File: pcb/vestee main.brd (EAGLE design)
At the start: 65 x 65 mm, 54 parts, among them IC1 LD117AS12TR, IC2 FT232RL, Q1 MMBT2222A, Q2 MMBT5088, Q3 MMBT4403, Q4 MMBT5088, Q5 MMBT5088

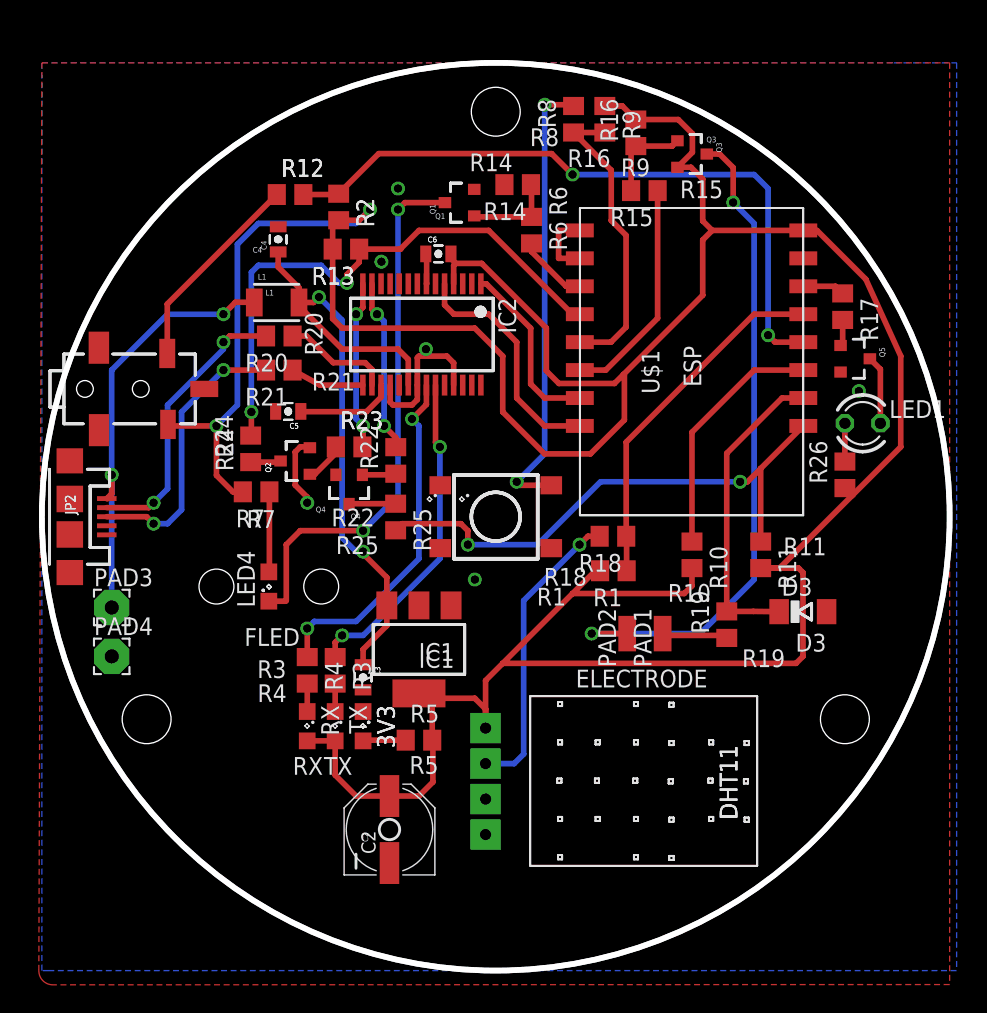
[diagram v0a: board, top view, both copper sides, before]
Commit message: Version 2, all issues fixed
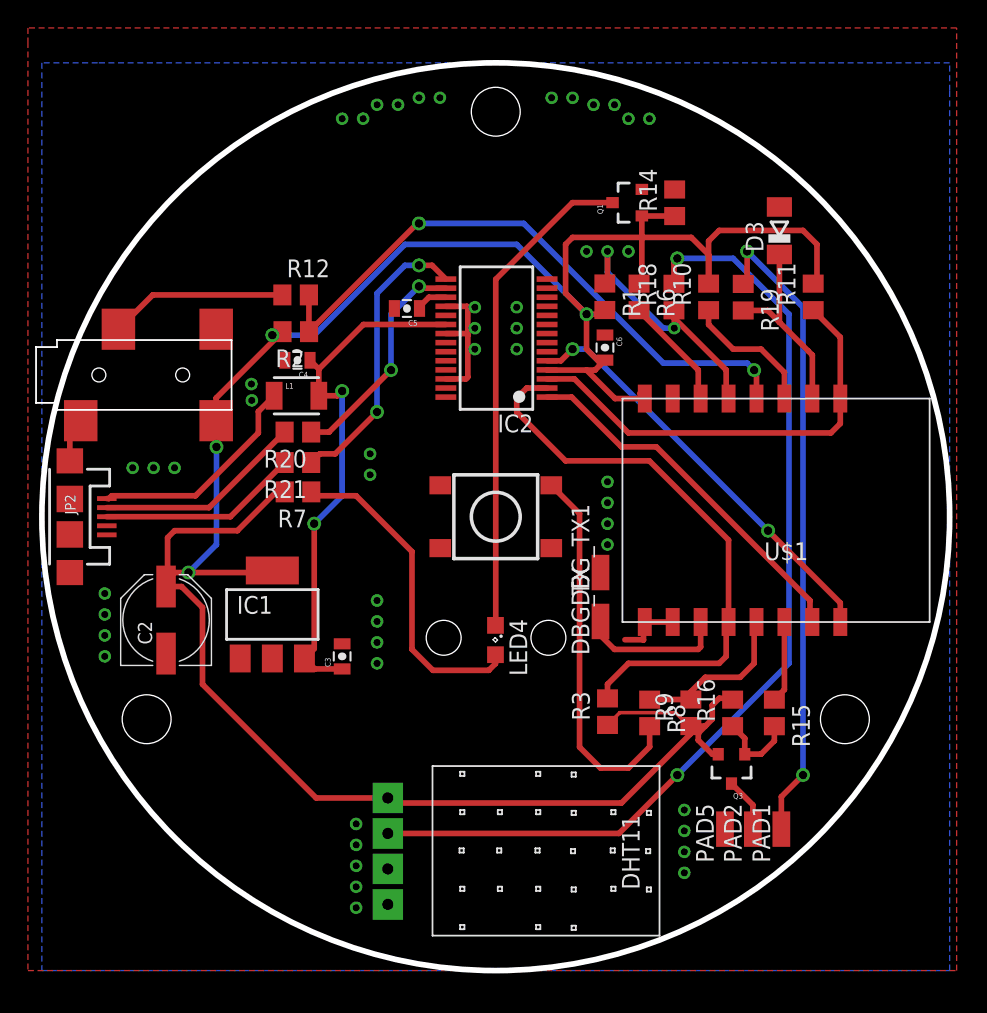
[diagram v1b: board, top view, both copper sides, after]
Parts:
- removed 3V3, RX, TX: (no value), led:SML0805
- removed LED1: (no value), led:LED3MM
- removed PAD3, PAD4: WIREPAD2,54/1,0, wirepad:2,54/1,0
- removed Q2, Q4, Q5: MMBT5088, SparkFun-DiscreteSemi:SOT23-3
- removed R13, R17, R22, R23, R24, R25, R26, R4, R5: (no value), rcl:R0805
- added DBG_TX, DBG_TX1, PAD5: (no value), wirepad:SMD1,27-2,54
- PRPIHERALS: value (none) -> AUDIO-JACK-2.5-CUI; device SparkFun-Connectors:STEREOJACK2.5MM -> SparkFun-Connectors:STEREOJACK2.5_SMD_CUI
- moved Q3 44.1 mm to (49.4, 14.5), turned to 180 degrees
- moved R9 42.9 mm to (46.5, 18.5), turned to 90 degrees
- moved R8 42.9 mm to (43.5, 18.4), turned to 270 degrees
- moved R16 42.1 mm to (49.5, 18.4)
- moved R15 38.5 mm to (52.5, 18.4), turned to 270 degrees
- moved D3 27.3 mm to (52.8, 53.0), turned to 90 degrees
- moved R19 23.5 mm to (50.2, 48.2), turned to 270 degrees
- moved C2 21.9 mm to (8.89, 25.1)
- moved R3 19.7 mm to (40.5, 18.5), turned to 90 degrees
- moved R1 19.6 mm to (40.3, 48.2), turned to 270 degrees
- moved R11 18.8 mm to (55.2, 48.2), turned to 90 degrees
- moved R10 18.5 mm to (47.7, 48.2), turned to 90 degrees
- moved R18 17.7 mm to (45.3, 48.2), turned to 90 degrees
- moved LED4 16.7 mm to (32.5, 23.7), turned to 270 degrees
- moved PAD2 16.6 mm to (50.9, 10.1)
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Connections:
- removed net CBUS: R13.1, R24.2, U$1.GPIO0
- removed net CBUS_RST: R11.1, R25.2, U$1.REST
- removed net N$11: IC2.23, R3.1
- removed net N$12: IC2.22, R4.1
- removed net N$13: R3.2, TX.C
- removed net N$14: R4.2, RX.C
- removed net N$20: R17.1, U$1.GPIO12
- removed net N$22: LED1.K, Q5.3
- removed net N$23: LED1.A, R26.2
- removed net N$30: IC2.13, R22.2
- removed net N$31: Q2.3, R24.1
- removed net N$32: Q2.1, R23.1
- removed net N$33: Q4.1, R22.1
- removed net N$34: IC2.14, R23.2
- removed net N$35: Q4.3, R25.1
- removed net N$8: 3V3.A, R5.1
- new net DTR: IC2.2, R3.2, U$1.GPIO0
- new net RTS: IC2.3, R11.1, U$1.REST
- net 1-WIRE: now also PRPIHERALS.3; no longer PRPIHERALS.1
- net FLED: now also U$1.GPIO12; no longer U$1.GPIO2
- net GND: now also DBG_TX1.1, PAD5.1, PRPIHERALS.1; no longer 3V3.C, PAD4.1, PRPIHERALS.5, Q2.2, Q4.2, Q5.2
- net N$5: now also DBG_TX.1, U$1.GPIO2; no longer Q5.1, R17.2
- net N$7: no longer PAD3.1
- net VCC: now also PRPIHERALS.2, R3.1; no longer PRPIHERALS.4, R13.2, R26.1, R5.2, RX.A, TX.A
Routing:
- net VCC: track 245.3 -> 182.1 mm, vias 2 -> 4
- net N$6: track 21.4 -> 70.4 mm, vias 1 -> 2
- net N$17: track 48.2 -> 3.89 mm, vias 2 -> 0
- net N$26: track 4.72 -> 46.1 mm, vias 0 -> 2
- net DTR: track 0.00 -> 41.2 mm
- net CBUS: track 40.9 -> 0.00 mm, vias 2 -> 0
- net CBUS_RST: track 39.3 -> 0.00 mm, vias 2 -> 0
- net RTS: track 0.00 -> 31.8 mm
- net N$12: track 25.2 -> 0.00 mm, vias 2 -> 0
- net N$11: track 23.6 -> 0.00 mm, vias 2 -> 0
- net N$15: track 5.75 -> 23.4 mm
- net N$28: track 5.31 -> 20.9 mm, vias 0 -> 2
- net N$7: track 31.2 -> 15.9 mm, vias 2 -> 0
- net FTDI_TXD: track 12.8 -> 26.5 mm
- net FTDI_RXD: track 17.1 -> 30.2 mm, vias 0 -> 2
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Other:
- board text removed: "/Users/grzegorz/Documents/montebmp.bmp"
- board text removed: "3V3"
- board text removed: "C2"
- board text removed: "C3"
- board text removed: "C4"
- board text removed: "C5"
- board text removed: "C6"
- board text removed: "D3"
- board text removed: "DHT11"
- board text removed: "ELECTRODE"
- board text removed: "ESP"
- board text removed: "FLED"
- board text removed: "IC1"
- board text removed: "JP2"
- board text removed: "L1"
- board text removed: "Q1"
- board text removed: "Q2"
- board text removed: "Q3"
- board text removed: "Q4"
- board text removed: "R1"
- board text removed: "R10"
- board text removed: "R11"
- board text removed: "R12"
- board text removed: "R13"
- board text removed: "R14"
- board text removed: "R15"
- board text removed: "R16"
- board text removed: "R18"
- board text removed: "R19"
- board text removed: "R2"
- board text removed: "R20"
- board text removed: "R21"
- board text removed: "R22"
- board text removed: "R23"
- board text removed: "R24"
- board text removed: "R25"
- board text removed: "R3"
- board text removed: "R4"
- board text removed: "R5"
- board text removed: "R6"
- board text removed: "R7"
- board text removed: "R8"
- board text removed: "R9"
- board text removed: "RX"
- board text removed: "TX"
- board text removed: "vestee"

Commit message: pcb rev3
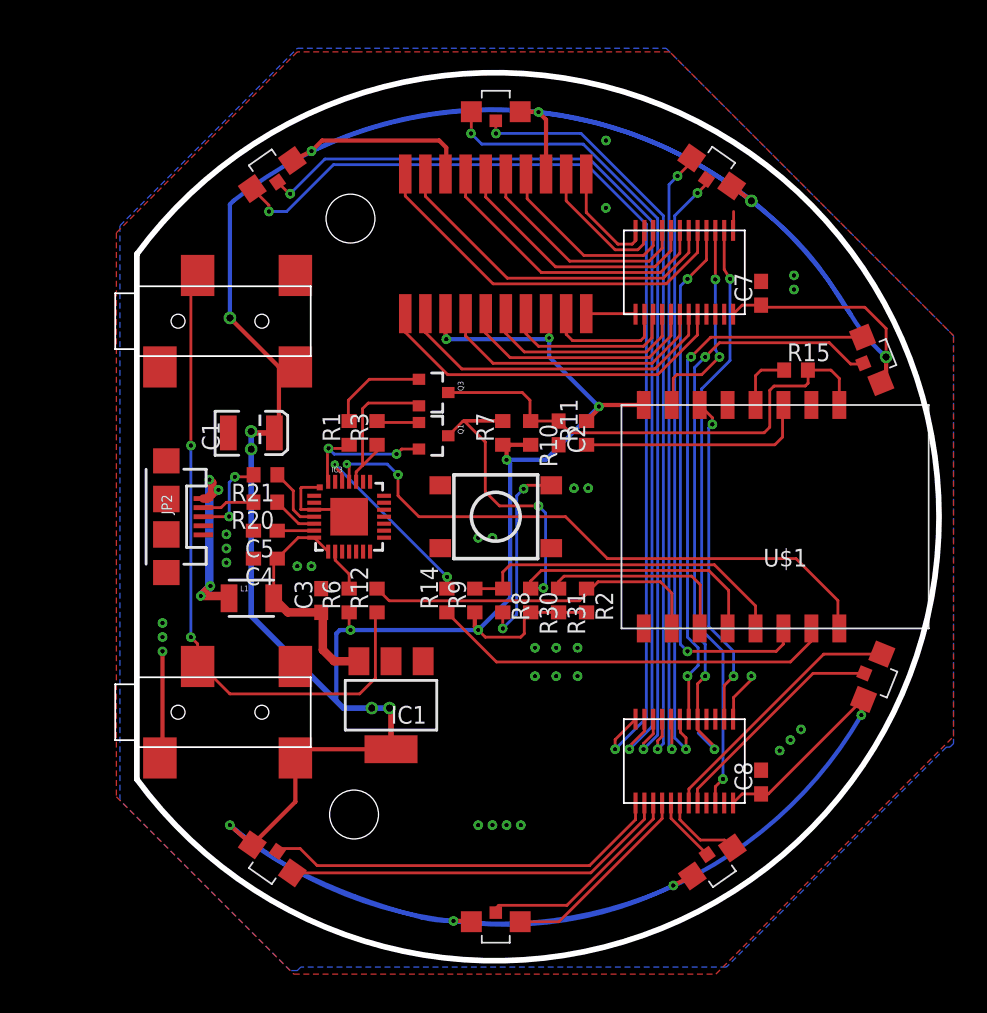
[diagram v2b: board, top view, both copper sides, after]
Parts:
- removed C6: 100nF, SparkFun-Capacitors:0805-CAP
- removed DBG_TX, DBG_TX1, PAD1, PAD2, PAD5: (no value), wirepad:SMD1,27-2,54
- removed IC2: FT232RL, ftdichip:SSOP28
- removed LED4: (no value), led:SML0805
- removed R16, R18, R19: (no value), rcl:R0805
- added C1: (no value), SparkFun-Passives:EIA3528
- added C7, C8: 100nF, rcl:C0603
- added D1, D2, D4, D5, D6, D7, D8: KPBA-3010ESGC, SparkFun-LED:APA3010SF4C
- added IC3: CP210X_USB_UART, SparkFun-DigitalIC:MLP28
- added PRPIHERALS1: AUDIO-JACK-2.5-CUI, SparkFun-Connectors:STEREOJACK2.5_SMD_CUI
- added R30, R31: 12k, rcl:R0603
- added U$3, U$4: SCT2024CSSG, vestee:SSOP24
- C2: value (none) -> 100nF; device SparkFun-Capacitors:PANASONIC_D -> rcl:C0603
- C3: device SparkFun-Capacitors:0805-CAP -> rcl:C0603
- C4: value 10nF -> 10n; device SparkFun-Capacitors:0805-CAP -> rcl:C0603
- C5: value 100nF -> 100n; device SparkFun-Capacitors:0805-CAP -> rcl:C0603
- D3: value (none) -> KPBA-3010ESGC; device diode:SOD80C -> SparkFun-LED:APA3010SF4C
- Q3: value MMBT4403 -> MMBT2222A
- R1, R12, R2, R20, R21, R3, R7: device rcl:R0805 -> rcl:R0603
- R10, R11, R6, R9: value (none) -> 12k; device rcl:R0805 -> rcl:R0603
- R14, R8: value (none) -> 470R; device rcl:R0805 -> rcl:R0603
- R15: value (none) -> 470; device rcl:R0805 -> rcl:R0603
- U$2: value (none) -> KCDA02-103; device DHT11:DHT11 -> vestee:KCDA02-103
- moved U$2 43.6 mm to (32.5, 52.0), turned to 0 degrees
- moved Q3 34.4 mm to (28.0, 41.4), turned to 270 degrees
- moved R14 32.8 mm to (29.0, 26.5)
- moved C2 31.1 mm to (37.0, 38.5), turned to 270 degrees
- moved R6 30.1 mm to (22.0, 26.5), turned to 90 degrees
- moved R2 28.4 mm to (39.0, 26.5), turned to 270 degrees
- moved R3 25.9 mm to (24.0, 38.5)
- moved R15 24.6 mm to (54.0, 43.0), turned to 0 degrees
- moved R12 22.6 mm to (24.0, 26.5), turned to 90 degrees
- moved Q1 21.8 mm to (28.0, 38.3), turned to 270 degrees
- moved R1 20.7 mm to (22.0, 38.5), turned to 90 degrees
- moved R11 18.9 mm to (39.0, 38.5)
- moved C5 18.9 mm to (16.0, 31.5)
- moved R9 17.4 mm to (31.0, 26.5)
- moved R10 16.0 mm to (35.0, 38.5), turned to 270 degrees
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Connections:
- net N$19 renamed SWITCH
- removed net ELECTRODE: R15.1, U$1.GPIO4
- removed net FLED: R6.2, U$1.GPIO12
- removed net N$1: R1.1, R18.1, U$1.GPIO14
- removed net N$10: Q1.1, R14.1, R6.1
- removed net N$16: LED4.C, Q1.3
- removed net N$17: PAD2.1, Q3.3
- removed net N$21: R10.1, U$1.CH_PD
- removed net N$26: PAD1.1, R19.1
- removed net N$27: Q3.1, R15.2, R16.1
- removed net N$4: R12.2, R2.1, U$1.GPIO16
- removed net N$6: R18.2, U$2.DATA
- new net A1: U$2.17, U$3.7
- new net A2: U$2.12, U$3.11
- new net B1: U$2.16, U$3.8
- new net B2: U$2.11, U$3.12
- new net C1: U$2.4, U$3.18
- new net C2: U$2.9, U$3.14
- new net CH_PD: R11.1, U$1.CH_PD
- new net CLK: U$1.GPIO13, U$3.3
- new net D1: U$2.2, U$3.19
- new net D1G: D1.3, U$4.12
- new net D1R: D1.2, U$4.11
- new net D2: U$2.7, U$3.15
- new net D2G: D2.3, U$4.10
- new net D2R: D2.2, U$4.9
- new net D3G: D3.3, U$4.8
- new net D3R: D3.2, U$4.7
- new net D4G: D4.3, U$4.6
- new net D4R: D4.2, U$4.5
- new net D5G: D5.3, U$4.19
- new net D5R: D5.2, U$4.20
- new net D6G: D6.3, U$4.18
- new net D6R: D6.2, U$4.17
- new net D7G: D7.3, U$4.16
- new net D7R: D7.2, U$4.15
- new net D8G: D8.3, U$4.14
- new net D8R: D8.2, U$4.13
- new net DP1: U$2.5, U$3.17
- new net DP2: U$2.10, U$3.13
- new net E1: U$2.1, U$3.20
- new net E2: U$2.6, U$3.16
- new net F1: U$2.19, U$3.6
- new net F2: U$2.14, U$3.10
- new net G1: U$2.20, U$3.5
- new net G2: U$2.15, U$3.9
- new net GPIO0: Q1.3, R30.1, R7.2, U$1.GPIO0
- new net GPIO16: R15.1, U$1.GPIO16
- new net GPIO2: R31.1, U$1.GPIO2
- new net JACK: PRPIHERALS.3, PRPIHERALS1.3, R12.1
- new net LA/: U$1.GPIO4, U$3.4
- new net N$14: IC3.9, R6.2
- new net REST: C2.1, Q3.3, R10.1, R15.2, U$1.REST
- new net SDI: U$1.GPIO12, U$4.2
- new net SDO: U$3.2, U$4.22
- new net TXD: IC3.26, R14.2
- net 1-WIRE: now also R12.2, R2.1, U$1.GPIO15; no longer PRPIHERALS.3, R12.1
- net ADC: no longer D3.C, R19.2
- net DTR: now also IC3.28, Q1.2, R1.1; no longer IC2.2, R3.2, U$1.GPIO0
- net FTDI_RXD: now also IC3.25; no longer IC2.5
- net FTDI_TXD: now also R14.1; no longer IC2.1
- net GND: now also C1.C, C2.2, C7.2, C8.2, IC3.3, IC3.EXP, IC3.M, PRPIHERALS1.1, U$3.1, U$4.1; no longer C2.-, C6.1, D3.A, DBG_TX1.1, IC2.18, IC2.21, IC2.25, IC2.26, IC2.7, PAD5.1, Q1.2, R14.2, U$1.GPIO15, U$2.GND
- net N$15: now also Q1.1, R3.2; no longer LED4.A, R7.1
- net N$28: now also IC3.4; no longer IC2.15
- net N$29: now also IC3.5; no longer IC2.16
- net N$5: now also Q3.1, R1.2; no longer DBG_TX.1, U$1.GPIO2
- net N$9: now also IC3.6; no longer IC2.17
- net RTS: now also IC3.24, Q3.2, R3.1; no longer IC2.3, R11.1, U$1.REST
- net VCC: now also C1.A, C7.1, C8.1, D1.COM, D2.COM, D3.COM, D4.COM, D5.COM, D6.COM, D7.COM, D8.COM, PRPIHERALS1.2, R30.2, R31.2, R6.1, R7.1, U$2.13, U$2.18, U$2.3, U$2.8, U$3.24, U$4.24; no longer C2.+, C6.2, IC2.4, Q3.2, R1.2, R16.2, R3.1, R7.2, U$2.VCC
- net VIN: now also IC3.7, IC3.8; no longer IC2.20
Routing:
- net VCC: track 182.1 -> 383.6 mm, vias 4 -> 19
- net D1G: track 0.00 -> 73.6 mm, vias 0 -> 2
- net D1R: track 0.00 -> 71.1 mm, vias 0 -> 2
- net N$6: track 70.4 -> 0.00 mm, vias 2 -> 0
- net D2G: track 0.00 -> 58.3 mm, vias 0 -> 2
- net D2R: track 0.00 -> 56.0 mm, vias 0 -> 2
- net JACK: track 0.00 -> 47.2 mm, vias 0 -> 2
- net N$26: track 46.1 -> 0.00 mm, vias 2 -> 0
- net D3G: track 0.00 -> 45.3 mm, vias 0 -> 2
- net D3R: track 0.00 -> 44.4 mm, vias 0 -> 2
- net N$4: track 44.2 -> 0.00 mm, vias 2 -> 0
- net D4R: track 0.00 -> 43.5 mm, vias 0 -> 3
- net SDO: track 0.00 -> 42.8 mm, vias 0 -> 2
- net GPIO0: track 0.00 -> 42.7 mm, vias 0 -> 2
- net D4G: track 0.00 -> 39.6 mm, vias 0 -> 2
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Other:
- board size 65 x 65 mm -> 57.4 x 63.6 mm
- board text removed: "and"
- board text removed: "vestee.io"
